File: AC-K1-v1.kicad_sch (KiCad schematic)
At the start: 170 parts, among them J1 S2B-PH-K-SLFSN, SW1 ESC, SW10 F9, SW11 F10, SW12 F11, SW13 F12, SW14 CARET, SW15 1, SW16 2, SW17 3, SW18 4, SW19 5, SW2 F1, SW20 6, SW21 7, SW22 8, SW23 9, SW24 0, SW25 ß, SW26 GRAVE, SW27 BSPC, SW28 DELETE, SW29 HOME, SW3 F2, SW30 TAB, SW31 Q, SW32 W, SW33 E, SW34 R, SW35 T, SW36 Z, SW37 U, SW38 I, SW39 O, SW4 F3, SW40 P, SW41 Ü, SW42 ASTRK, SW43 ENTER, SW44 PG_UP, SW45 LCTRL, SW46 A, SW47 S, SW48 D, SW49 F, SW5 F4, SW50 G, SW51 H, SW52 J, SW53 K, SW54 L, SW55 Ö, SW56 Ä, SW57 HASH, SW58 PG_DN, SW59 LSHIFT, SW6 F5, SW60 LT, SW61 Y, SW62 X, SW63 C, SW64 V, SW65 B, SW66 N, SW67 M, SW68 COMMA, SW69 DOT, SW7 F6, SW70 MINUS, SW71 RSHIFT, SW72 UP, SW73 END, SW74 LCTRL, SW75 LCMD, SW76 LALT, SW77 SPACE, SW78 RALT, SW79 FN, SW8 F7, SW80 RCTRL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

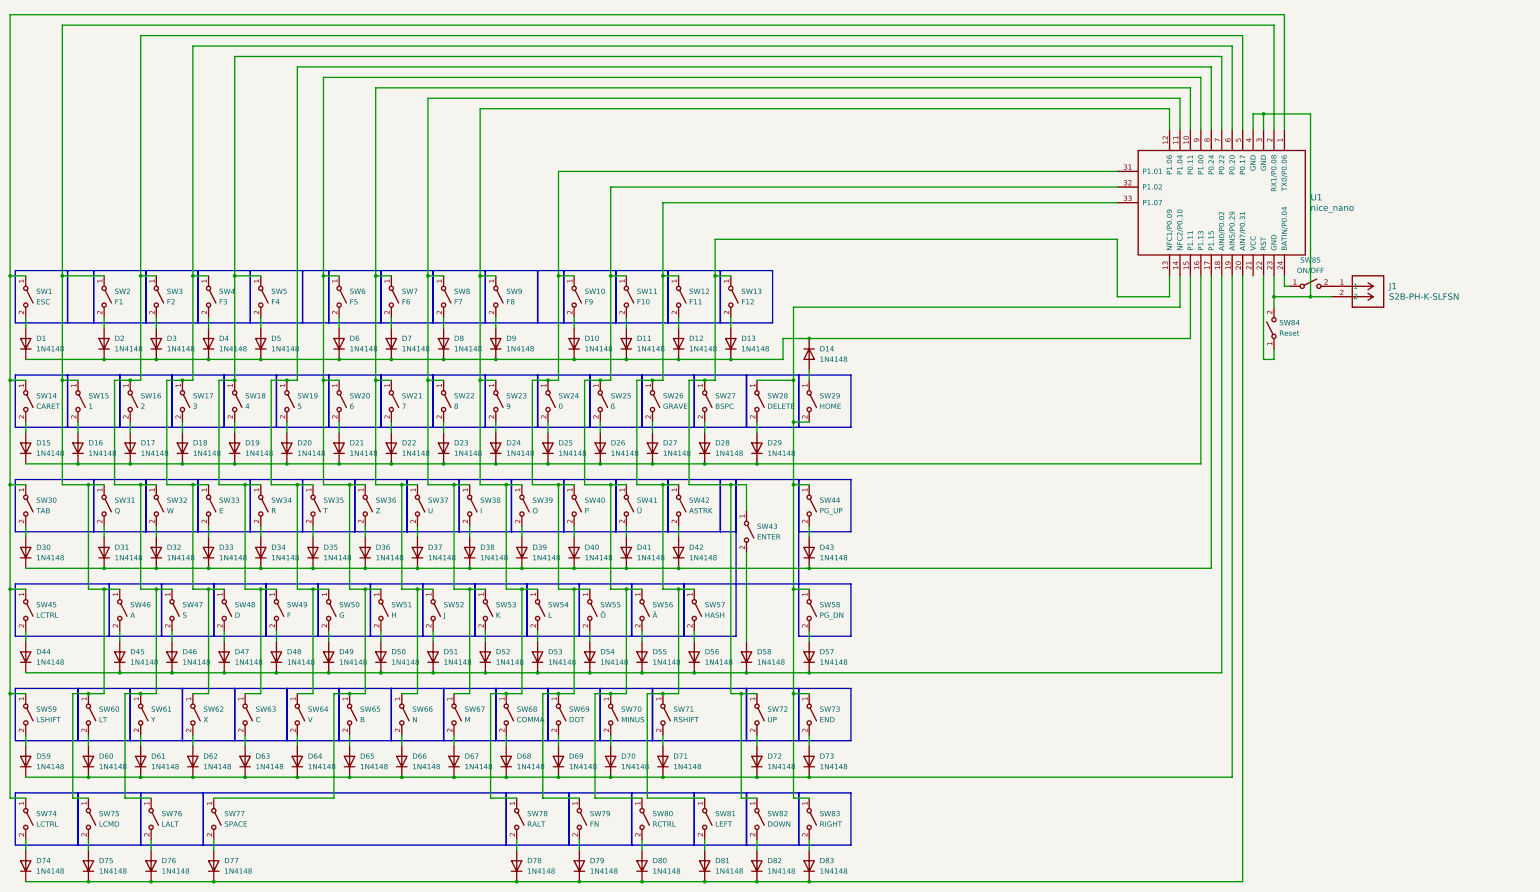
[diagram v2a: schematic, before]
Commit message: Redoing everything
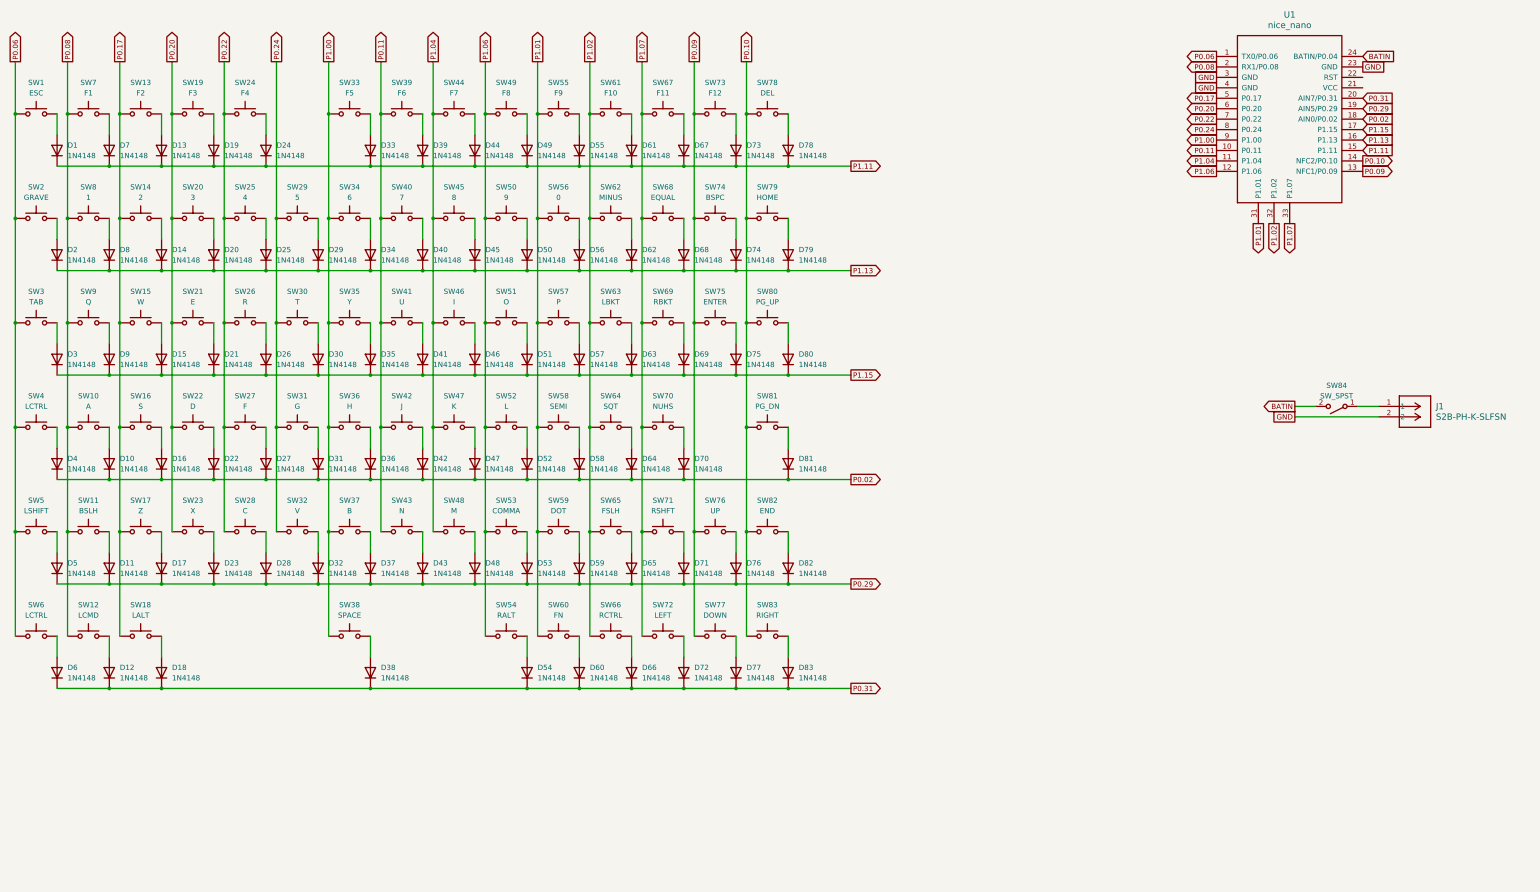
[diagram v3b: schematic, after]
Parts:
- removed SW1: ESC, Switch_Keyboard_Kailh:SW_Kailh_Choc_V1V2_1.00u, symbol Switch:SW_SPST
- removed SW10: F9, Switch_Keyboard_Kailh:SW_Kailh_Choc_V1V2_1.00u, symbol Switch:SW_SPST
- removed SW11: F10, Switch_Keyboard_Kailh:SW_Kailh_Choc_V1V2_1.00u, symbol Switch:SW_SPST
- removed SW12: F11, Switch_Keyboard_Kailh:SW_Kailh_Choc_V1V2_1.00u, symbol Switch:SW_SPST
- removed SW13: F12, Switch_Keyboard_Kailh:SW_Kailh_Choc_V1V2_1.00u, symbol Switch:SW_SPST
- removed SW14: CARET, Switch_Keyboard_Kailh:SW_Kailh_Choc_V1V2_1.00u, symbol Switch:SW_SPST
- removed SW15: 1, Switch_Keyboard_Kailh:SW_Kailh_Choc_V1V2_1.00u, symbol Switch:SW_SPST
- removed SW16: 2, Switch_Keyboard_Kailh:SW_Kailh_Choc_V1V2_1.00u, symbol Switch:SW_SPST
- removed SW17: 3, Switch_Keyboard_Kailh:SW_Kailh_Choc_V1V2_1.00u, symbol Switch:SW_SPST
- removed SW18: 4, Switch_Keyboard_Kailh:SW_Kailh_Choc_V1V2_1.00u, symbol Switch:SW_SPST
- removed SW19: 5, Switch_Keyboard_Kailh:SW_Kailh_Choc_V1V2_1.00u, symbol Switch:SW_SPST
- removed SW2: F1, Switch_Keyboard_Kailh:SW_Kailh_Choc_V1V2_1.00u, symbol Switch:SW_SPST
- removed SW20: 6, Switch_Keyboard_Kailh:SW_Kailh_Choc_V1V2_1.00u, symbol Switch:SW_SPST
- removed SW21: 7, Switch_Keyboard_Kailh:SW_Kailh_Choc_V1V2_1.00u, symbol Switch:SW_SPST
- removed SW22: 8, Switch_Keyboard_Kailh:SW_Kailh_Choc_V1V2_1.00u, symbol Switch:SW_SPST
- removed SW23: 9, Switch_Keyboard_Kailh:SW_Kailh_Choc_V1V2_1.00u, symbol Switch:SW_SPST
- removed SW24: 0, Switch_Keyboard_Kailh:SW_Kailh_Choc_V1V2_1.00u, symbol Switch:SW_SPST
- removed SW25: ß, Switch_Keyboard_Kailh:SW_Kailh_Choc_V1V2_1.00u, symbol Switch:SW_SPST
- removed SW26: GRAVE, Switch_Keyboard_Kailh:SW_Kailh_Choc_V1V2_1.00u, symbol Switch:SW_SPST
- removed SW27: BSPC, Switch_Keyboard_Kailh:SW_Kailh_Choc_V1V2_1.00u, symbol Switch:SW_SPST
- removed SW28: DELETE, Switch_Keyboard_Kailh:SW_Kailh_Choc_V1V2_1.00u, symbol Switch:SW_SPST
- removed SW29: HOME, Switch_Keyboard_Kailh:SW_Kailh_Choc_V1V2_1.00u, symbol Switch:SW_SPST
- removed SW3: F2, Switch_Keyboard_Kailh:SW_Kailh_Choc_V1V2_1.00u, symbol Switch:SW_SPST
- removed SW30: TAB, Switch_Keyboard_Kailh:SW_Kailh_Choc_V1V2_1.50u, symbol Switch:SW_SPST
- removed SW31: Q, Switch_Keyboard_Kailh:SW_Kailh_Choc_V1V2_1.00u, symbol Switch:SW_SPST
- removed SW32: W, Switch_Keyboard_Kailh:SW_Kailh_Choc_V1V2_1.00u, symbol Switch:SW_SPST
- removed SW33: E, Switch_Keyboard_Kailh:SW_Kailh_Choc_V1V2_1.00u, symbol Switch:SW_SPST
- removed SW34: R, Switch_Keyboard_Kailh:SW_Kailh_Choc_V1V2_1.00u, symbol Switch:SW_SPST
- removed SW35: T, Switch_Keyboard_Kailh:SW_Kailh_Choc_V1V2_1.00u, symbol Switch:SW_SPST
- removed SW36: Z, Switch_Keyboard_Kailh:SW_Kailh_Choc_V1V2_1.00u, symbol Switch:SW_SPST
- removed SW37: U, Switch_Keyboard_Kailh:SW_Kailh_Choc_V1V2_1.00u, symbol Switch:SW_SPST
- removed SW38: I, Switch_Keyboard_Kailh:SW_Kailh_Choc_V1V2_1.00u, symbol Switch:SW_SPST
- removed SW39: O, Switch_Keyboard_Kailh:SW_Kailh_Choc_V1V2_1.00u, symbol Switch:SW_SPST
- removed SW4: F3, Switch_Keyboard_Kailh:SW_Kailh_Choc_V1V2_1.00u, symbol Switch:SW_SPST
- removed SW40: P, Switch_Keyboard_Kailh:SW_Kailh_Choc_V1V2_1.00u, symbol Switch:SW_SPST
- removed SW41: Ü, Switch_Keyboard_Kailh:SW_Kailh_Choc_V1V2_1.00u, symbol Switch:SW_SPST
- removed SW42: ASTRK, Switch_Keyboard_Kailh:SW_Kailh_Choc_V1V2_1.00u, symbol Switch:SW_SPST
- removed SW43: ENTER, Switch_Keyboard_Kailh:SW_Kailh_Choc_V1V2_ISOEnter, symbol Switch:SW_SPST
- removed SW44: PG_UP, Switch_Keyboard_Kailh:SW_Kailh_Choc_V1V2_1.00u, symbol Switch:SW_SPST
- removed SW45: LCTRL, Switch_Keyboard_Kailh:SW_Kailh_Choc_V1V2_1.75u, symbol Switch:SW_SPST
- removed SW46: A, Switch_Keyboard_Kailh:SW_Kailh_Choc_V1V2_1.00u, symbol Switch:SW_SPST
- removed SW47: S, Switch_Keyboard_Kailh:SW_Kailh_Choc_V1V2_1.00u, symbol Switch:SW_SPST
- removed SW48: D, Switch_Keyboard_Kailh:SW_Kailh_Choc_V1V2_1.00u, symbol Switch:SW_SPST
- removed SW49: F, Switch_Keyboard_Kailh:SW_Kailh_Choc_V1V2_1.00u, symbol Switch:SW_SPST
- removed SW5: F4, Switch_Keyboard_Kailh:SW_Kailh_Choc_V1V2_1.00u, symbol Switch:SW_SPST
- removed SW50: G, Switch_Keyboard_Kailh:SW_Kailh_Choc_V1V2_1.00u, symbol Switch:SW_SPST
- removed SW51: H, Switch_Keyboard_Kailh:SW_Kailh_Choc_V1V2_1.00u, symbol Switch:SW_SPST
- removed SW52: J, Switch_Keyboard_Kailh:SW_Kailh_Choc_V1V2_1.00u, symbol Switch:SW_SPST
- removed SW53: K, Switch_Keyboard_Kailh:SW_Kailh_Choc_V1V2_1.00u, symbol Switch:SW_SPST
- removed SW54: L, Switch_Keyboard_Kailh:SW_Kailh_Choc_V1V2_1.00u, symbol Switch:SW_SPST
- removed SW55: Ö, Switch_Keyboard_Kailh:SW_Kailh_Choc_V1V2_1.00u, symbol Switch:SW_SPST
- removed SW56: Ä, Switch_Keyboard_Kailh:SW_Kailh_Choc_V1V2_1.00u, symbol Switch:SW_SPST
- removed SW57: HASH, Switch_Keyboard_Kailh:SW_Kailh_Choc_V1V2_1.00u, symbol Switch:SW_SPST
- removed SW58: PG_DN, Switch_Keyboard_Kailh:SW_Kailh_Choc_V1V2_1.00u, symbol Switch:SW_SPST
- removed SW59: LSHIFT, Switch_Keyboard_Kailh:SW_Kailh_Choc_V1V2_1.25u, symbol Switch:SW_SPST
- removed SW6: F5, Switch_Keyboard_Kailh:SW_Kailh_Choc_V1V2_1.00u, symbol Switch:SW_SPST
- removed SW60: LT, Switch_Keyboard_Kailh:SW_Kailh_Choc_V1V2_1.00u, symbol Switch:SW_SPST
- removed SW61: Y, Switch_Keyboard_Kailh:SW_Kailh_Choc_V1V2_1.00u, symbol Switch:SW_SPST
- removed SW62: X, Switch_Keyboard_Kailh:SW_Kailh_Choc_V1V2_1.00u, symbol Switch:SW_SPST
- removed SW63: C, Switch_Keyboard_Kailh:SW_Kailh_Choc_V1V2_1.00u, symbol Switch:SW_SPST
- removed SW64: V, Switch_Keyboard_Kailh:SW_Kailh_Choc_V1V2_1.00u, symbol Switch:SW_SPST
- removed SW65: B, Switch_Keyboard_Kailh:SW_Kailh_Choc_V1V2_1.00u, symbol Switch:SW_SPST
- removed SW66: N, Switch_Keyboard_Kailh:SW_Kailh_Choc_V1V2_1.00u, symbol Switch:SW_SPST
- removed SW67: M, Switch_Keyboard_Kailh:SW_Kailh_Choc_V1V2_1.00u, symbol Switch:SW_SPST
- removed SW68: COMMA, Switch_Keyboard_Kailh:SW_Kailh_Choc_V1V2_1.00u, symbol Switch:SW_SPST
- removed SW69: DOT, Switch_Keyboard_Kailh:SW_Kailh_Choc_V1V2_1.00u, symbol Switch:SW_SPST
- removed SW7: F6, Switch_Keyboard_Kailh:SW_Kailh_Choc_V1V2_1.00u, symbol Switch:SW_SPST
- removed SW70: MINUS, Switch_Keyboard_Kailh:SW_Kailh_Choc_V1V2_1.00u, symbol Switch:SW_SPST
- removed SW71: RSHIFT, Switch_Keyboard_Kailh:SW_Kailh_Choc_V1V2_1.75u, symbol Switch:SW_SPST
- removed SW72: UP, Switch_Keyboard_Kailh:SW_Kailh_Choc_V1V2_1.00u, symbol Switch:SW_SPST
- removed SW73: END, Switch_Keyboard_Kailh:SW_Kailh_Choc_V1V2_1.00u, symbol Switch:SW_SPST
- removed SW74: LCTRL, Switch_Keyboard_Kailh:SW_Kailh_Choc_V1V2_1.25u, symbol Switch:SW_SPST
- removed SW75: LCMD, Switch_Keyboard_Kailh:SW_Kailh_Choc_V1V2_1.25u, symbol Switch:SW_SPST
- removed SW76: LALT, Switch_Keyboard_Kailh:SW_Kailh_Choc_V1V2_1.25u, symbol Switch:SW_SPST
- removed SW77: SPACE, Switch_Keyboard_Kailh:SW_Kailh_Choc_V1V2_5.50u, symbol Switch:SW_SPST
- removed SW78: RALT, Switch_Keyboard_Kailh:SW_Kailh_Choc_V1V2_1.25u, symbol Switch:SW_SPST
- removed SW79: FN, Switch_Keyboard_Kailh:SW_Kailh_Choc_V1V2_1.25u, symbol Switch:SW_SPST
- removed SW8: F7, Switch_Keyboard_Kailh:SW_Kailh_Choc_V1V2_1.00u, symbol Switch:SW_SPST
- removed SW80: RCTRL, Switch_Keyboard_Kailh:SW_Kailh_Choc_V1V2_1.25u, symbol Switch:SW_SPST
- removed SW81: LEFT, Switch_Keyboard_Kailh:SW_Kailh_Choc_V1V2_1.00u, symbol Switch:SW_SPST
- removed SW82: DOWN, Switch_Keyboard_Kailh:SW_Kailh_Choc_V1V2_1.00u, symbol Switch:SW_SPST
- removed SW83: RIGHT, Switch_Keyboard_Kailh:SW_Kailh_Choc_V1V2_1.00u, symbol Switch:SW_SPST
- removed SW85: ON/OFF, Switch_Keyboard_Kailh:SW_Kailh_Choc_V1V2_1.00u, symbol Switch:SW_SPST
- removed SW9: F8, Switch_Keyboard_Kailh:SW_Kailh_Choc_V1V2_1.00u, symbol Switch:SW_SPST
- added SW1: ESC, marbastlib-choc:SW_choc_v1_1u, symbol Switch:SW_Push
- added SW10: A, marbastlib-choc:SW_choc_v1_1u, symbol Switch:SW_Push
- added SW11: BSLH, marbastlib-choc:SW_choc_v1_1u, symbol Switch:SW_Push
- added SW12: LCMD, marbastlib-choc:SW_choc_v1_1.25u, symbol Switch:SW_Push
- added SW13: F2, marbastlib-choc:SW_choc_v1_1u, symbol Switch:SW_Push
- added SW14: 2, marbastlib-choc:SW_choc_v1_1u, symbol Switch:SW_Push
- added SW15: W, marbastlib-choc:SW_choc_v1_1u, symbol Switch:SW_Push
- added SW16: S, marbastlib-choc:SW_choc_v1_1u, symbol Switch:SW_Push
- added SW17: Z, marbastlib-choc:SW_choc_v1_1u, symbol Switch:SW_Push
- added SW18: LALT, marbastlib-choc:SW_choc_v1_1.25u, symbol Switch:SW_Push
- added SW19: F3, marbastlib-choc:SW_choc_v1_1u, symbol Switch:SW_Push
- added SW2: GRAVE, marbastlib-choc:SW_choc_v1_1u, symbol Switch:SW_Push
- added SW20: 3, marbastlib-choc:SW_choc_v1_1u, symbol Switch:SW_Push
- added SW21: E, marbastlib-choc:SW_choc_v1_1u, symbol Switch:SW_Push
- added SW22: D, marbastlib-choc:SW_choc_v1_1u, symbol Switch:SW_Push
- added SW23: X, marbastlib-choc:SW_choc_v1_1u, symbol Switch:SW_Push
- added SW24: F4, marbastlib-choc:SW_choc_v1_1u, symbol Switch:SW_Push
- added SW25: 4, marbastlib-choc:SW_choc_v1_1u, symbol Switch:SW_Push
- added SW26: R, marbastlib-choc:SW_choc_v1_1u, symbol Switch:SW_Push
- added SW27: F, marbastlib-choc:SW_choc_v1_1u, symbol Switch:SW_Push
- added SW28: C, marbastlib-choc:SW_choc_v1_1u, symbol Switch:SW_Push
- added SW29: 5, marbastlib-choc:SW_choc_v1_1u, symbol Switch:SW_Push
- added SW3: TAB, marbastlib-choc:SW_choc_v1_1.5u, symbol Switch:SW_Push
- added SW30: T, marbastlib-choc:SW_choc_v1_1u, symbol Switch:SW_Push
- added SW31: G, marbastlib-choc:SW_choc_v1_1u, symbol Switch:SW_Push
- added SW32: V, marbastlib-choc:SW_choc_v1_1u, symbol Switch:SW_Push
- added SW33: F5, marbastlib-choc:SW_choc_v1_1u, symbol Switch:SW_Push
- added SW34: 6, marbastlib-choc:SW_choc_v1_1u, symbol Switch:SW_Push
- added SW35: Y, marbastlib-choc:SW_choc_v1_1u, symbol Switch:SW_Push
- added SW36: H, marbastlib-choc:SW_choc_v1_1u, symbol Switch:SW_Push
- added SW37: B, marbastlib-choc:SW_choc_v1_1u, symbol Switch:SW_Push
- added SW38: SPACE, Switch_Keyboard_Kailh:SW_Kailh_Choc_V1_6.00u, symbol Switch:SW_Push
- added SW39: F6, marbastlib-choc:SW_choc_v1_1u, symbol Switch:SW_Push
- added SW4: LCTRL, marbastlib-choc:SW_choc_v1_1.75u, symbol Switch:SW_Push
- added SW40: 7, marbastlib-choc:SW_choc_v1_1u, symbol Switch:SW_Push
- added SW41: U, marbastlib-choc:SW_choc_v1_1u, symbol Switch:SW_Push
- added SW42: J, marbastlib-choc:SW_choc_v1_1u, symbol Switch:SW_Push
- added SW43: N, marbastlib-choc:SW_choc_v1_1u, symbol Switch:SW_Push
- added SW44: F7, marbastlib-choc:SW_choc_v1_1u, symbol Switch:SW_Push
- added SW45: 8, marbastlib-choc:SW_choc_v1_1u, symbol Switch:SW_Push
- added SW46: I, marbastlib-choc:SW_choc_v1_1u, symbol Switch:SW_Push
- added SW47: K, marbastlib-choc:SW_choc_v1_1u, symbol Switch:SW_Push
- added SW48: M, marbastlib-choc:SW_choc_v1_1u, symbol Switch:SW_Push
- added SW49: F8, marbastlib-choc:SW_choc_v1_1u, symbol Switch:SW_Push
- added SW5: LSHIFT, marbastlib-choc:SW_choc_v1_1.25u, symbol Switch:SW_Push
- added SW50: 9, marbastlib-choc:SW_choc_v1_1u, symbol Switch:SW_Push
- added SW51: O, marbastlib-choc:SW_choc_v1_1u, symbol Switch:SW_Push
- added SW52: L, marbastlib-choc:SW_choc_v1_1u, symbol Switch:SW_Push
- added SW53: COMMA, marbastlib-choc:SW_choc_v1_1u, symbol Switch:SW_Push
- added SW54: RALT, marbastlib-choc:SW_choc_v1_1.25u, symbol Switch:SW_Push
- added SW55: F9, marbastlib-choc:SW_choc_v1_1u, symbol Switch:SW_Push
- added SW56: 0, marbastlib-choc:SW_choc_v1_1u, symbol Switch:SW_Push
- added SW57: P, marbastlib-choc:SW_choc_v1_1u, symbol Switch:SW_Push
- added SW58: SEMI, marbastlib-choc:SW_choc_v1_1u, symbol Switch:SW_Push
- added SW59: DOT, marbastlib-choc:SW_choc_v1_1u, symbol Switch:SW_Push
- added SW6: LCTRL, marbastlib-choc:SW_choc_v1_1.25u, symbol Switch:SW_Push
- added SW60: FN, marbastlib-choc:SW_choc_v1_1.25u, symbol Switch:SW_Push
- added SW61: F10, marbastlib-choc:SW_choc_v1_1u, symbol Switch:SW_Push
- added SW62: MINUS, marbastlib-choc:SW_choc_v1_1u, symbol Switch:SW_Push
- added SW63: LBKT, marbastlib-choc:SW_choc_v1_1u, symbol Switch:SW_Push
- added SW64: SQT, marbastlib-choc:SW_choc_v1_1u, symbol Switch:SW_Push
- added SW65: FSLH, marbastlib-choc:SW_choc_v1_1u, symbol Switch:SW_Push
- added SW66: RCTRL, marbastlib-choc:SW_choc_v1_1.25u, symbol Switch:SW_Push
- added SW67: F11, marbastlib-choc:SW_choc_v1_1u, symbol Switch:SW_Push
- added SW68: EQUAL, marbastlib-choc:SW_choc_v1_1u, symbol Switch:SW_Push
- added SW69: RBKT, marbastlib-choc:SW_choc_v1_1u, symbol Switch:SW_Push
- added SW7: F1, marbastlib-choc:SW_choc_v1_1u, symbol Switch:SW_Push
- added SW70: NUHS, marbastlib-choc:SW_choc_v1_1u, symbol Switch:SW_Push
- added SW71: RSHFT, marbastlib-choc:SW_choc_v1_1.75u, symbol Switch:SW_Push
- added SW72: LEFT, marbastlib-choc:SW_choc_v1_1u, symbol Switch:SW_Push
- added SW73: F12, marbastlib-choc:SW_choc_v1_1u, symbol Switch:SW_Push
- added SW74: BSPC, marbastlib-choc:SW_choc_v1_1u, symbol Switch:SW_Push
- added SW75: ENTER, Switch_Keyboard_Kailh:SW_Kailh_Choc_V1_ISOEnter, symbol Switch:SW_Push
- added SW76: UP, marbastlib-choc:SW_choc_v1_1u, symbol Switch:SW_Push
- added SW77: DOWN, marbastlib-choc:SW_choc_v1_1u, symbol Switch:SW_Push
- added SW78: DEL, marbastlib-choc:SW_choc_v1_1u, symbol Switch:SW_Push
- added SW79: HOME, marbastlib-choc:SW_choc_v1_1u, symbol Switch:SW_Push
- added SW8: 1, marbastlib-choc:SW_choc_v1_1u, symbol Switch:SW_Push
- added SW80: PG_UP, marbastlib-choc:SW_choc_v1_1u, symbol Switch:SW_Push
- added SW81: PG_DN, marbastlib-choc:SW_choc_v1_1u, symbol Switch:SW_Push
- added SW82: END, marbastlib-choc:SW_choc_v1_1u, symbol Switch:SW_Push
- added SW83: RIGHT, marbastlib-choc:SW_choc_v1_1u, symbol Switch:SW_Push
- added SW9: Q, marbastlib-choc:SW_choc_v1_1u, symbol Switch:SW_Push
- SW84: value Reset -> SW_SPST; footprint Button_Switch_THT:SW_PUSH_1P1T_6x3.5mm_H4.3_APEM_MJTP1243 -> Button_Switch_THT:SW_Slide_SPDT_Angled_CK_OS102011MA1Q
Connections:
- net at D35.2 (A): now also SW35.2
- net P0.08: now reaches U1.2 (RX1/P0.08)
- net P0.08: now also SW10.1, SW11.1, SW12.1, SW7.1, SW8.1, SW9.1
- net at D31.2 (A): now also SW31.2
- net at D62.2 (A): now also SW62.2
- net P1.00: now reaches U1.9 (P1.00)
- net P1.00: now also SW33.1, SW34.1, SW35.1, SW36.1, SW37.1, SW38.1
- net at D65.2 (A): now also SW65.2
- net at D39.2 (A): now also SW39.2
- net at D26.2 (A): now also SW26.2
- net P1.04: now reaches U1.11 (P1.04)
- net P1.04: now also SW44.1, SW45.1, SW46.1, SW47.1, SW48.1
- net at D8.2 (A): now also SW8.2
- net P0.11: now reaches U1.10 (P0.11)
- net P0.11: now also SW39.1, SW40.1, SW41.1, SW42.1, SW43.1
- net at D22.2 (A): now also SW22.2
- net P0.20: now reaches U1.6 (P0.20)
- net P0.20: now also SW19.1, SW20.1, SW21.1, SW22.1, SW23.1
- net at D4.2 (A): now also SW4.2
- net P0.10: now reaches U1.14 (NFC2/P0.10)
- net P0.10: now also SW78.1, SW79.1, SW80.1, SW81.1, SW82.1, SW83.1
- net at D29.2 (A): now also SW29.2
- net at D2.2 (A): now also SW2.2
- net at D59.2 (A): now also SW59.2
- net P0.24: now reaches U1.8 (P0.24)
- net P0.24: now also SW29.1, SW30.1, SW31.1, SW32.1
- net at D49.2 (A): now also SW49.2
- net at D14.2 (A): now also SW14.2
- net at D58.2 (A): now also SW58.2
- net P0.09: now reaches U1.13 (NFC1/P0.09)
- net P0.09: now also SW73.1, SW74.1, SW75.1, SW76.1, SW77.1
- net at D13.2 (A): now also SW13.2
- net P1.07: now reaches U1.33 (P1.07)
- net P1.07: now also SW67.1, SW68.1, SW69.1, SW70.1, SW71.1, SW72.1
- net at D12.2 (A): now also SW12.2
- net at D7.2 (A): now also SW7.2
- net at D37.2 (A): now also SW37.2
- net at D50.2 (A): now also SW50.2
- net at D43.2 (A): now also SW43.2
- net at D32.2 (A): now also SW32.2
- net at D6.2 (A): now also SW6.2
- net at D83.2 (A): now also SW83.2
- net at D33.2 (A): now also SW33.2
- net at D25.2 (A): now also SW25.2
- net at SW84.1 (A): now also J1.1; no longer U1.22 (RST)
- net GND: now reaches J1.2, U1.23 (GND), U1.3 (GND), U1.4 (GND)
- net GND: no longer SW84.2 (B)
- net at D9.2 (A): now also SW9.2
- net at D21.2 (A): now also SW21.2
- net P1.06: now reaches U1.12 (P1.06)
- net P1.06: now also SW49.1, SW50.1, SW51.1, SW52.1, SW53.1, SW54.1
- net at D78.2 (A): now also SW78.2
- net at D57.2 (A): now also SW57.2
- net at D16.2 (A): now also SW16.2
- net at D60.2 (A): now also SW60.2
- net at D15.2 (A): now also SW15.2
- net at D70.2 (A): now also SW70.2
- net at D42.2 (A): now also SW42.2
- net at D63.2 (A): now also SW63.2
- net P1.01: now reaches U1.31 (P1.01)
- net P1.01: now also SW55.1, SW56.1, SW57.1, SW58.1, SW59.1, SW60.1
- net at D79.2 (A): now also SW79.2
- net at D20.2 (A): now also SW20.2
- net P0.17: now reaches U1.5 (P0.17)
- net P0.17: now also SW13.1, SW14.1, SW15.1, SW16.1, SW17.1, SW18.1
- net at D61.2 (A): now also SW61.2
- net at D67.2 (A): now also SW67.2
- net at D66.2 (A): now also SW66.2
- net P1.02: now reaches U1.32 (P1.02)
- net P1.02: now also SW61.1, SW62.1, SW63.1, SW64.1, SW65.1, SW66.1
- net at D11.2 (A): now also SW11.2
- net at D10.2 (A): now also SW10.2
- net at D54.2 (A): now also SW54.2
- net at D41.2 (A): now also SW41.2
- net at D69.2 (A): now also SW69.2
- net P0.22: now reaches U1.7 (P0.22)
- net P0.22: now also SW24.1, SW25.1, SW26.1, SW27.1, SW28.1
- net at D19.2 (A): now also SW19.2
- net at D71.2 (A): now also SW71.2
- net P0.06: now reaches U1.1 (TX0/P0.06)
- net P0.06: now also SW1.1, SW2.1, SW3.1, SW4.1, SW5.1, SW6.1
- net at D1.2 (A): now also SW1.2
- net at D73.2 (A): now also SW73.2
- net at D55.2 (A): now also SW55.2
- net at D18.2 (A): now also SW18.2
- net at D34.2 (A): now also SW34.2
- net at D36.2 (A): now also SW36.2
- net at D23.2 (A): now also SW23.2
- net at D80.2 (A): now also SW80.2
- net at D5.2 (A): now also SW5.2
- net at D68.2 (A): now also SW68.2
- net at D76.2 (A): now also SW76.2
- net at D28.2 (A): now also SW28.2
- net at D52.2 (A): now also SW52.2
- net BATIN: now reaches U1.24 (BATIN/P0.04)
- net BATIN: now also SW84.2 (B)
- net at D75.2 (A): now also SW75.2
- net at D27.2 (A): now also SW27.2
- net at D82.2 (A): now also SW82.2
- net at D17.2 (A): now also SW17.2
- net at D74.2 (A): now also SW74.2
- net at D53.2 (A): now also SW53.2
- net at D24.2 (A): now also SW24.2
- net at D45.2 (A): now also SW45.2
- net at D44.2 (A): now also SW44.2
- net at D48.2 (A): now also SW48.2
- net at D30.2 (A): now also SW30.2
- net at D38.2 (A): now also SW38.2
- net at D81.2 (A): now also SW81.2
- net at D77.2 (A): now also SW77.2
- net at D47.2 (A): now also SW47.2
- net at D64.2 (A): now also SW64.2
- net at D40.2 (A): now also SW40.2
- net at D72.2 (A): now also SW72.2
- net at D51.2 (A): now also SW51.2
- net at D56.2 (A): now also SW56.2
- net at D3.2 (A): now also SW3.2
- net at D46.2 (A): now also SW46.2
- new net P0.02: D10.1 (K), D16.1 (K), D22.1 (K), D27.1 (K), D31.1 (K), D36.1 (K), D4.1 (K), D42.1 (K), D47.1 (K), D52.1 (K), D58.1 (K), D64.1 (K), D70.1 (K), D81.1 (K), U1.18 (AIN0/P0.02)
- new net P0.29: D11.1 (K), D17.1 (K), D23.1 (K), D28.1 (K), D32.1 (K), D37.1 (K), D43.1 (K), D48.1 (K), D5.1 (K), D53.1 (K), D59.1 (K), D65.1 (K), D71.1 (K), D76.1 (K), D82.1 (K), U1.19 (AIN5/P0.29)
- new net P0.31: D12.1 (K), D18.1 (K), D38.1 (K), D54.1 (K), D6.1 (K), D60.1 (K), D66.1 (K), D72.1 (K), D77.1 (K), D83.1 (K), U1.20 (AIN7/P0.31)
- new net P1.11: D1.1 (K), D13.1 (K), D19.1 (K), D24.1 (K), D33.1 (K), D39.1 (K), D44.1 (K), D49.1 (K), D55.1 (K), D61.1 (K), D67.1 (K), D7.1 (K), D73.1 (K), D78.1 (K), U1.15 (P1.11)
- new net P1.13: D14.1 (K), D2.1 (K), D20.1 (K), D25.1 (K), D29.1 (K), D34.1 (K), D40.1 (K), D45.1 (K), D50.1 (K), D56.1 (K), D62.1 (K), D68.1 (K), D74.1 (K), D79.1 (K), D8.1 (K), U1.16 (P1.13)
- new net P1.15: D15.1 (K), D21.1 (K), D26.1 (K), D3.1 (K), D30.1 (K), D35.1 (K), D41.1 (K), D46.1 (K), D51.1 (K), D57.1 (K), D63.1 (K), D69.1 (K), D75.1 (K), D80.1 (K), D9.1 (K), U1.17 (P1.15)
